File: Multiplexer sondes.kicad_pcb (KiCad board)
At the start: 4 copper layers, 68.6 x 53.3 mm, 28 parts, among them J1 Conn_Coaxial, J2 DB9_Female_MountingHoles, K0 REED_1C, K1 REED_1C, K10 Reed_1A, K11 REED_1C, K111 REED_1C, K112 REED_1C, K12 REED_1C, K121 REED_1C, K122 REED_1C, K2 REED_1C, K20 Reed_1A, K21 REED_1C, K211 REED_1C, K212 REED_1C, K22 REED_1C, K221 REED_1C, K222 REED_1C, K30 Reed_1A, K40 Reed_1A

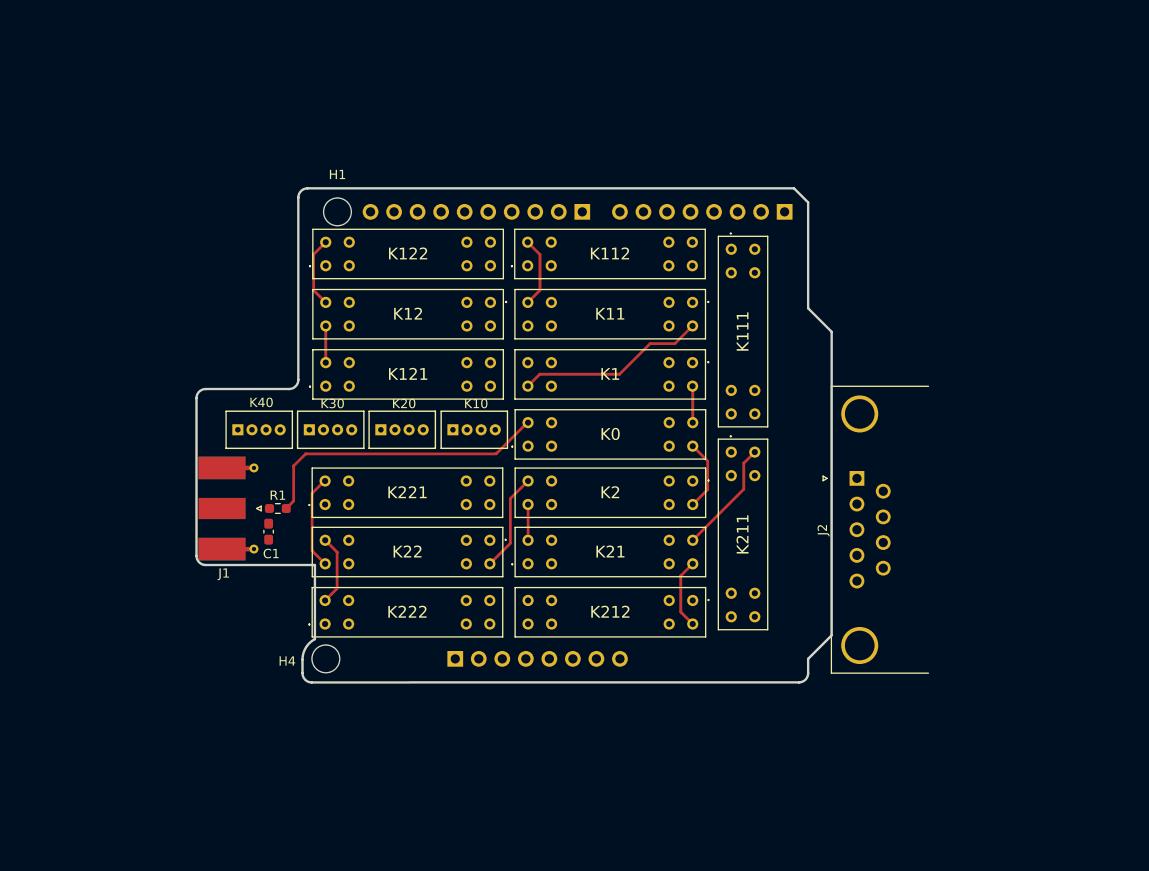
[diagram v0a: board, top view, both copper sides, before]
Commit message: v0.0 routed
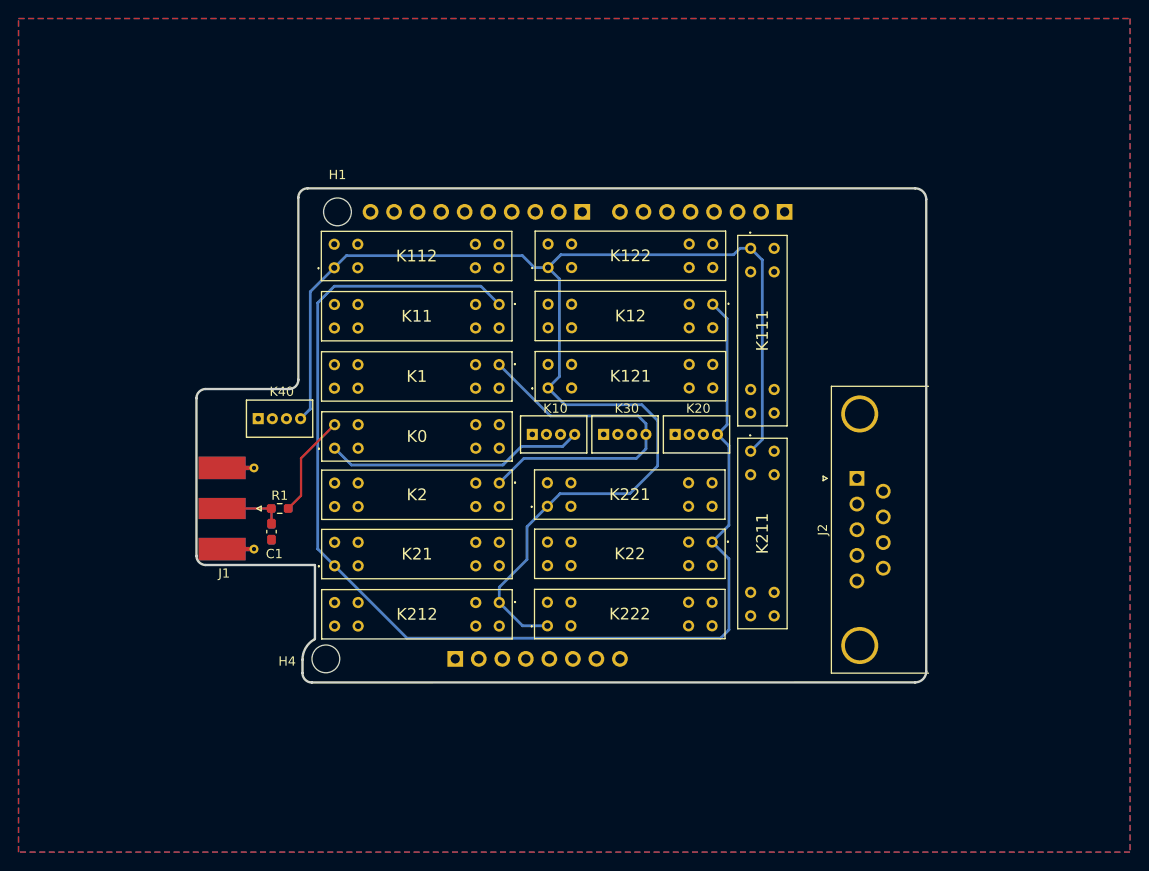
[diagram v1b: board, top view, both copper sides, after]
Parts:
- moved K20 31.8 mm to (165.9, 104.9)
- moved K30 31.8 mm to (158.2, 104.9)
- moved K12 24.0 mm to (169.9, 90.8)
- moved K121 24.0 mm to (152.2, 99.9)
- moved K122 24.0 mm to (152.2, 86.9)
- moved K22 24.0 mm to (169.9, 116.5)
- moved K221 24.0 mm to (152.1, 112.7)
- moved K222 24.0 mm to (152.1, 125.6)
- moved K0 20.9 mm to (129.1, 106.4)
- moved K1 20.9 mm to (146.9, 97.4)
- moved K11 20.9 mm to (146.9, 90.9)
- moved K112 20.9 mm to (129.1, 86.9)
- moved K2 20.9 mm to (146.9, 110.1)
- moved K21 20.9 mm to (129.1, 119.1)
- moved K212 20.9 mm to (146.9, 123.0)
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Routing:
- net /C4: track 0.00 -> 152.3 mm
- net /C3: track 0.00 -> 134.7 mm
- net /S4: track 0.00 -> 88.7 mm
- net /S3: track 0.00 -> 60.2 mm
- net /1to16_reedRelay/1to4_reedRelay4/S12: track 0.00 -> 52.9 mm
- net /S8: track 0.00 -> 52.0 mm
- net /1to16_reedRelay/S5-8: track 0.00 -> 50.9 mm
- net /1to16_reedRelay/S13-16: track 10.6 -> 51.5 mm
- net /C2: track 0.00 -> 38.6 mm
- net /S7: track 0.00 -> 38.2 mm
- net /S5: track 0.00 -> 37.0 mm
- net /S6: track 0.00 -> 35.2 mm
- net /C1: track 0.00 -> 28.0 mm
- net /1to16_reedRelay/1to4_reedRelay7/S12: track 12.3 -> 36.0 mm
- net /1to16_reedRelay/1to4_reedRelay5/S1234: track 32.3 -> 11.1 mm
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- added copper zone on In2.Cu, net /+5V_Ard_1
- added copper zone on B.Cu, net GND
- added copper zone on F.Cu, net GND
- added copper zone on In1.Cu, net GND
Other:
- board size 68.6 x 53.3 mm -> 78.8 x 53.3 mm
